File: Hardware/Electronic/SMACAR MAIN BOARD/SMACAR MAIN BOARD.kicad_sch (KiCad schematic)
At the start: 8 parts, among them J2 Conn_01x02, U2 ESP32-S3-DevKitC

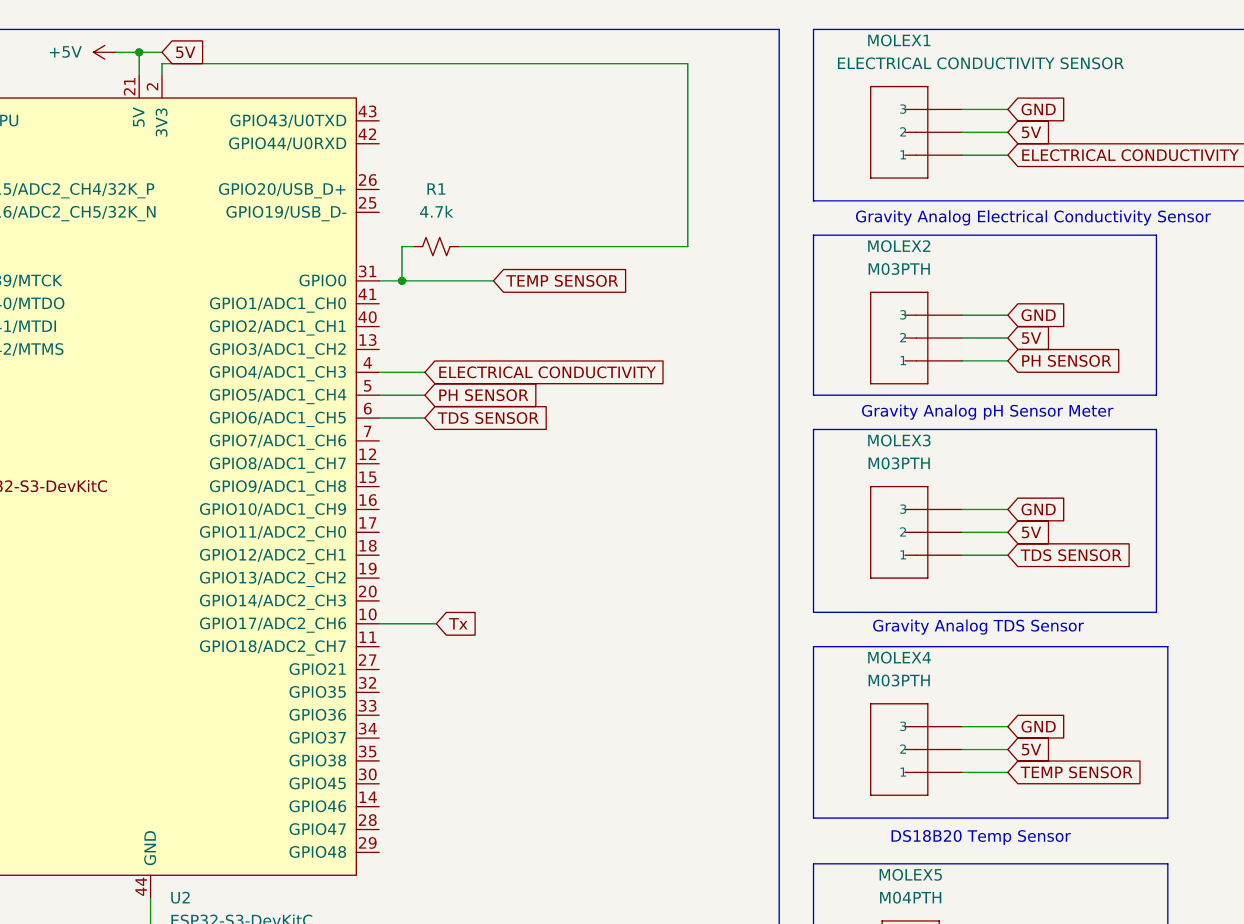
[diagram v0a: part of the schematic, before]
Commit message: PCBS
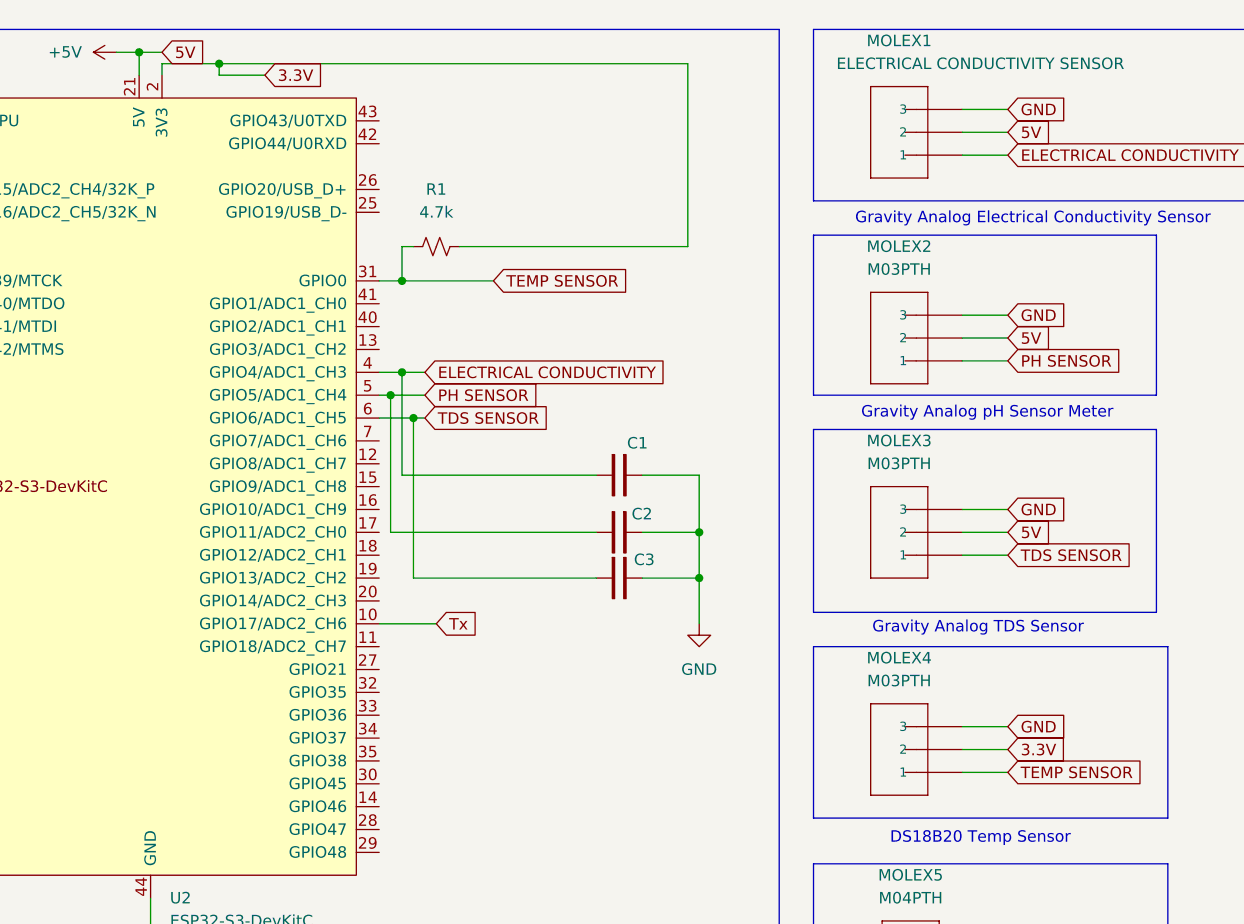
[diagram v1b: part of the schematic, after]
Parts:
- added C1, C2, C3: 100nF_Ceramic, Capacitor_THT:C_Disc_D5.0mm_W2.5mm_P2.50mm, symbol PCM_SL_Capacitors:100nF_Ceramic
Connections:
- net +5V: no longer MOLEX4.2
- net ELECTRICAL CONDUCTIVITY: now also C1.1
- net GND: now also C1.2, C2.2, C3.2
- net PH SENSOR: now also C2.1
- net TDS SENSOR: now also C3.1
- net 3.3V: now reaches R1.2, U2.1 (3V3), U2.2 (3V3)
- net 3.3V: now also MOLEX4.2
